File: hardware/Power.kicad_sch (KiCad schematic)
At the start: 0 parts

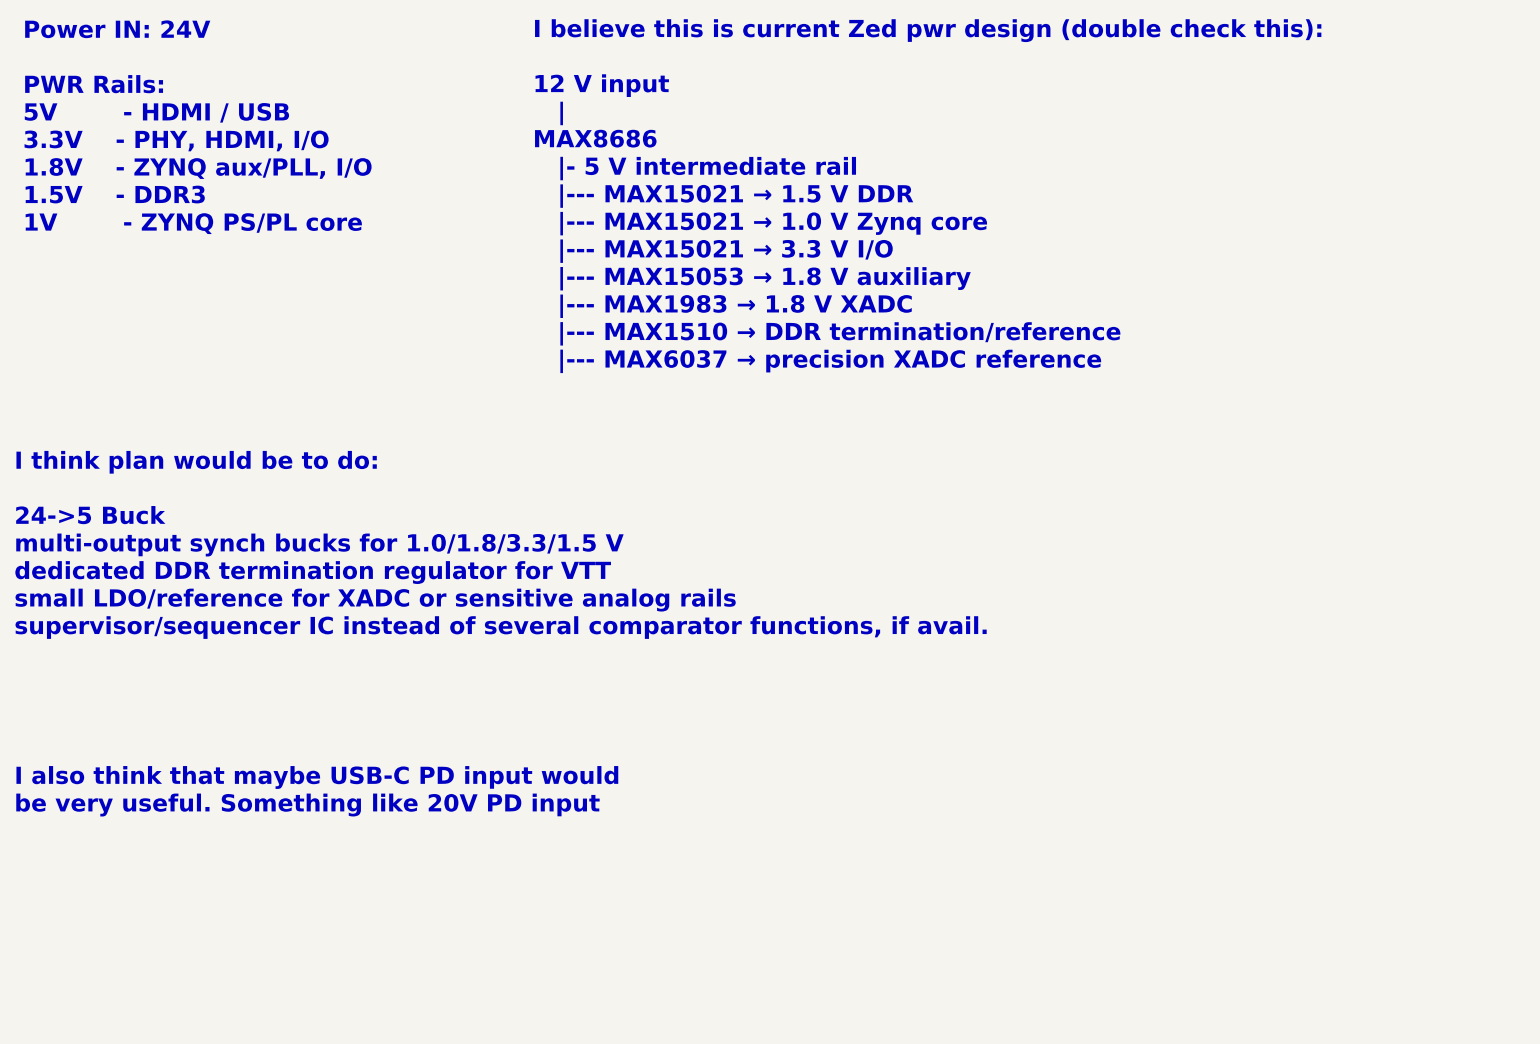
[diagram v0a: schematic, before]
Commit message: poop
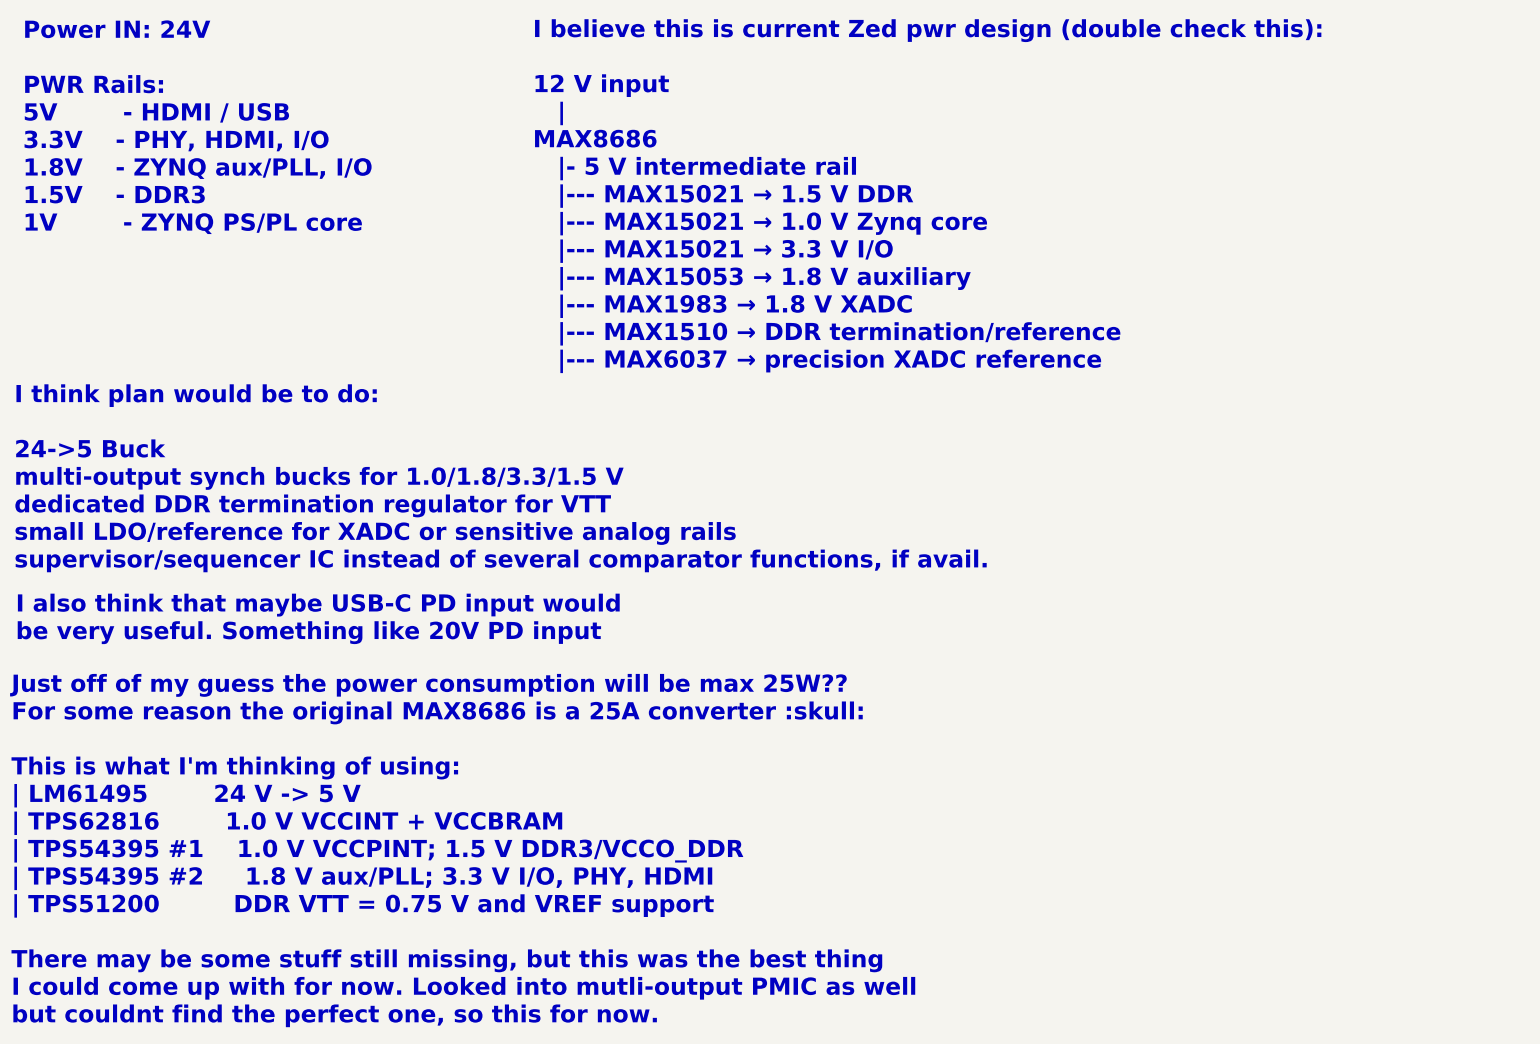
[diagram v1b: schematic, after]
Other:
- note added: "Just off of my guess the power consumption will be max 25W?? For some reason the original MAX8686 is a 25A converter :skull: This is what I'm thinking of using: | LM61495 24 V -> 5 V | TPS62816 1.0 V VCCINT + VCCBRAM | TPS54395 #1 1.0 V VCCPINT; 1.5 V DDR3/VCCO_DDR | TPS54395 #2 1.8 V aux/PLL; 3.3 V I/O, PHY, HDMI | TPS51200 DDR VTT = 0.75 V and VREF support There may be some stuff still missing,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"
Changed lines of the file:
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@@
 	(generator_version "10.0")
 	(paper "A4")
+	(text "Just off of my guess the power consumption will be max 25W??\nFor some reason the original MAX8686 is a 25A converter :skull:\n\nThis is what I'm thinking of using:\n| LM61495		24 V -> 5 V\n| TPS62816		1.0 V VCCINT + VCCBRAM\n| TPS54395 #1	1.0 V VCCPINT; 1.5 V DDR3/VCCO_DDR\n| TPS54395 #2 	1.8 V aux/PLL; 3.3 V I/O, PHY, HDMI\n| TPS51200 		DDR VTT = 0.75 V and VREF support\n\nThere may be some stuff still missing, but this was the best thing\nI could come up with for now. Looked into mutli-output PMIC as well\nbut couldnt find the perfect one, so this for now."
+		(exclude_from_sim no)
+		(at 18.796 164.084 0)
+		(effects
+			(font
+				(size 3 3)
+				(thickness 0.6)
+				(bold yes)
+			)
+			(justify left)
+		)
+	)
 	(text "Power IN: 24V\n\nPWR Rails:\n5V		- HDMI / USB\n3.3V	- PHY, HDMI, I/O\n1.8V	- ZYNQ aux/PLL, I/O\n1.5V	- DDR3\n1V		- ZYNQ PS/PL core"
 		(exclude_from_sim no)
@@
 	(text "I think plan would be to do:\n\n24->5 Buck\nmulti-output synch bucks for 1.0/1.8/3.3/1.5 V\ndedicated DDR termination regulator for VTT\nsmall LDO/reference for XADC or sensitive analog rails\nsupervisor/sequencer IC instead of several comparator functions, if avail."
 		(exclude_from_sim no)
-		(at 19.304 110.49 0)
+		(at 19.304 98.806 0)
 		(effects
 			(font
@@
 	(text "I also think that maybe USB-C PD input would\nbe very useful. Something like 20V PD input"
 		(exclude_from_sim no)
-		(at 19.304 153.67 0)
+		(at 19.558 123.444 0)
 		(effects
 			(font
